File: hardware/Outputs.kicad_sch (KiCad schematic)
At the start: 0 parts

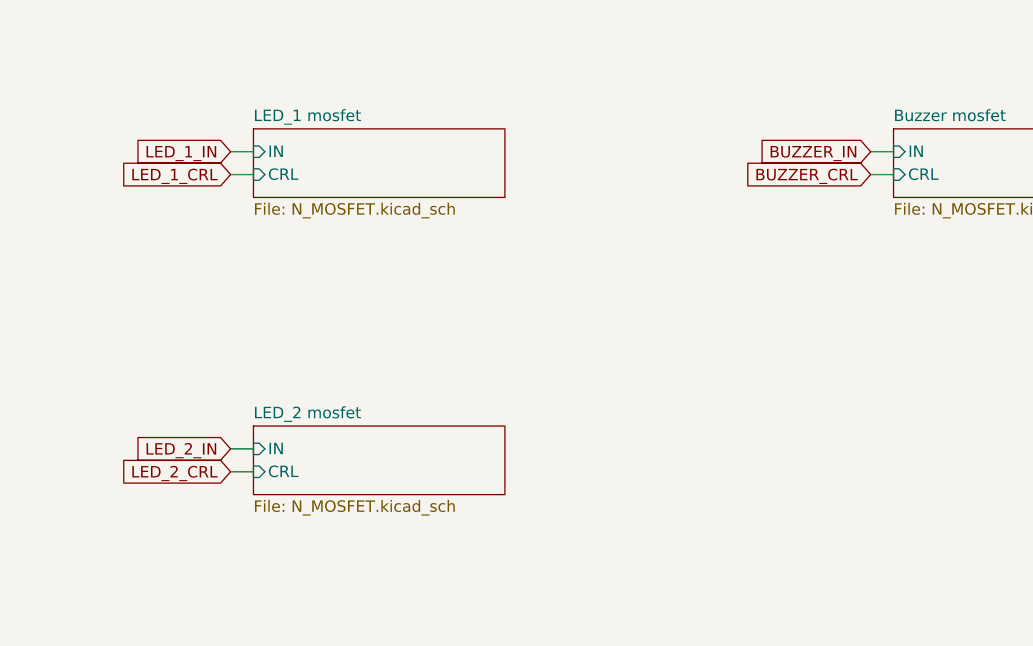
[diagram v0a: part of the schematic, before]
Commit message: changed some footprints for clarity, and made some progress on board
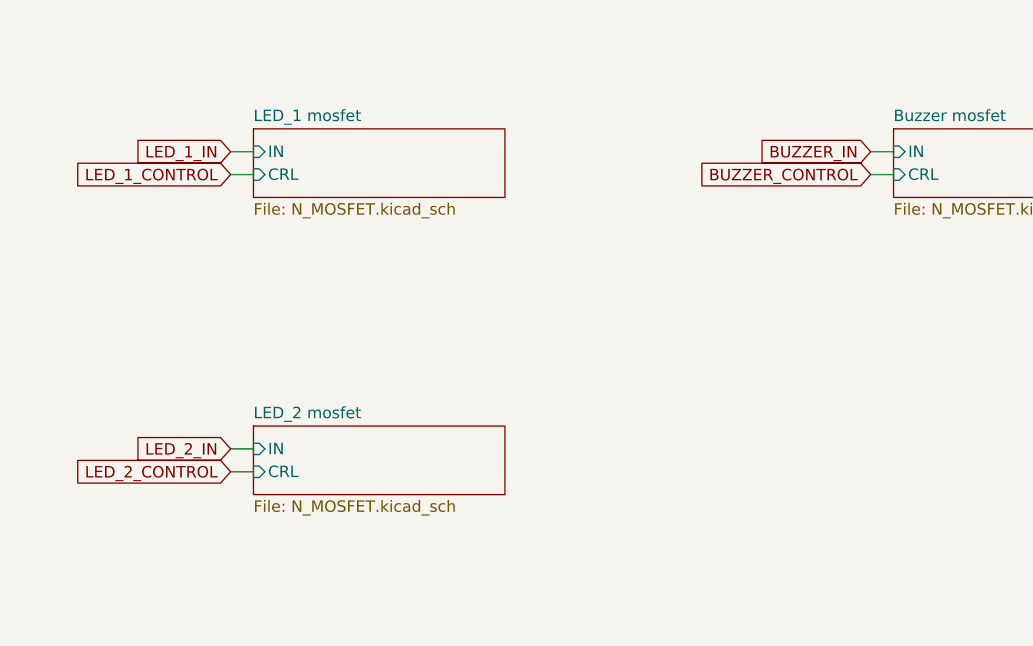
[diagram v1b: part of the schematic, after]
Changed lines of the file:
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@@
+    )
+  )
+  (global_label "BUZZER_CONTROL" (shape input) (at 120.015 109.22 180) (fields_autoplaced)
+    (effects (font (size 1.27 1.27)) (justify right))
+    (property "Intersheet References" "${INTERSHEET_REFS}" (id 0) (at 395.605 262.89 0)
+      (effects (font (size 1.27 1.27)) hide)
+    )
+  )
+  (global_label "LED_1_CONTROL" (shape input) (at 48.895 109.22 180) (fields_autoplaced)
+    (effects (font (size 1.27 1.27)) (justify right))
+    (property "Intersheet References" "${INTERSHEET_REFS}" (id 0) (at 324.485 257.81 0)
+      (effects (font (size 1.27 1.27)) hide)
     )
   )
@@
     )
   )
-  (global_label "LED_2_CRL" (shape input) (at 48.895 142.24 180) (fields_autoplaced)
-    (effects (font (size 1.27 1.27)) (justify right))
-    (property "Intersheet References" "${INTERSHEET_REFS}" (id 0) (at 36.4108 142.1606 0)
-      (effects (font (size 1.27 1.27)) (justify right) hide)
-    )
-  )
   (global_label "RTDS_GATE" (shape input) (at 120.015 80.645 180) (fields_autoplaced)
     (effects (font (size 1.27 1.27)) (justify right))
     (property "Intersheet References" "${INTERSHEET_REFS}" (id 0) (at -95.885 37.465 0)
+      (effects (font (size 1.27 1.27)) hide)
+    )
+  )
+  (global_label "LED_2_CONTROL" (shape input) (at 48.895 142.24 180) (fields_autoplaced)
+    (effects (font (size 1.27 1.27)) (justify right))
+    (property "Intersheet References" "${INTERSHEET_REFS}" (id 0) (at 324.485 288.29 0)
       (effects (font (size 1.27 1.27)) hide)
     )
@@
     )
   )
-  (global_label "BUZZER_CRL" (shape input) (at 120.015 109.22 180) (fields_autoplaced)
-    (effects (font (size 1.27 1.27)) (justify right))
-    (property "Intersheet References" "${INTERSHEET_REFS}" (id 0) (at 105.7165 109.1406 0)
-      (effects (font (size 1.27 1.27)) (justify right) hide)
-    )
-  )
-  (global_label "LED_1_CRL" (shape input) (at 48.895 109.22 180) (fields_autoplaced)
-    (effects (font (size 1.27 1.27)) (justify right))
-    (property "Intersheet References" "${INTERSHEET_REFS}" (id 0) (at 36.4108 109.1406 0)
-      (effects (font (size 1.27 1.27)) (justify right) hide)
-    )
-  )
